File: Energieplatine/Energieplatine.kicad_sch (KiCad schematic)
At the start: 22 parts, among them J1 USB_C_Receptacle_PowerOnly_6P, J2 Conn_01x02_Pin, U1 4027, U2 TL072, U3 LM2576HVT-ADJ, U4 LM2577T-ADJ

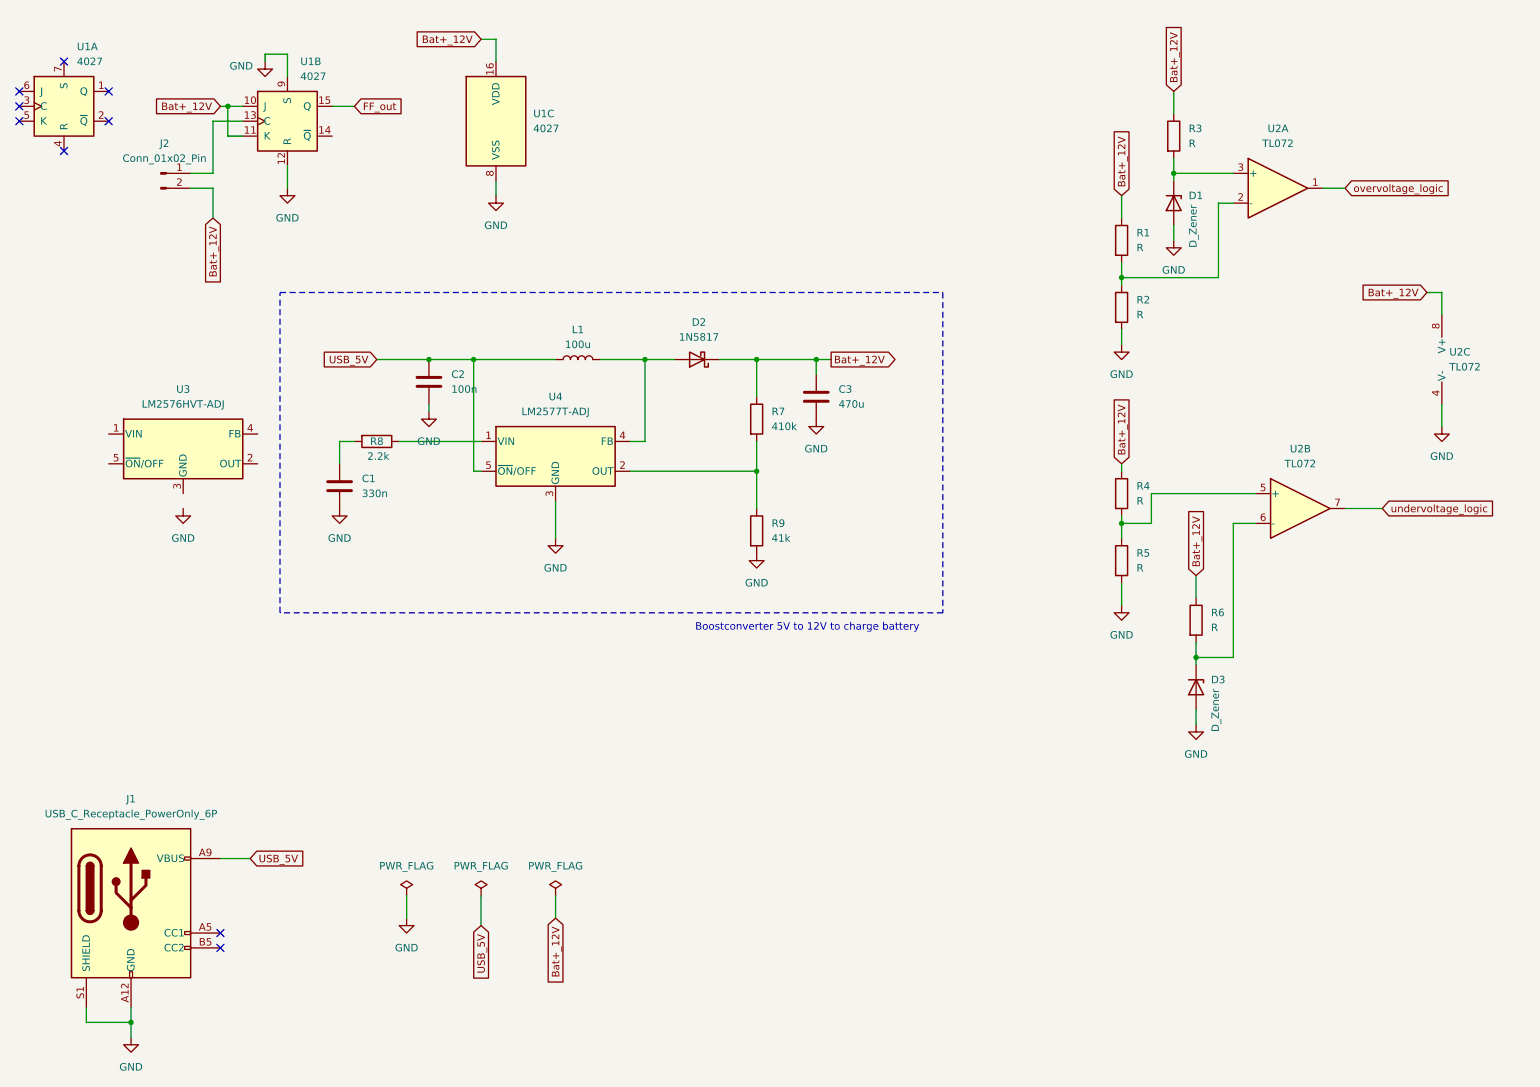
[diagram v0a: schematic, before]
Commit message: Update Energieplatine.kicad_sch
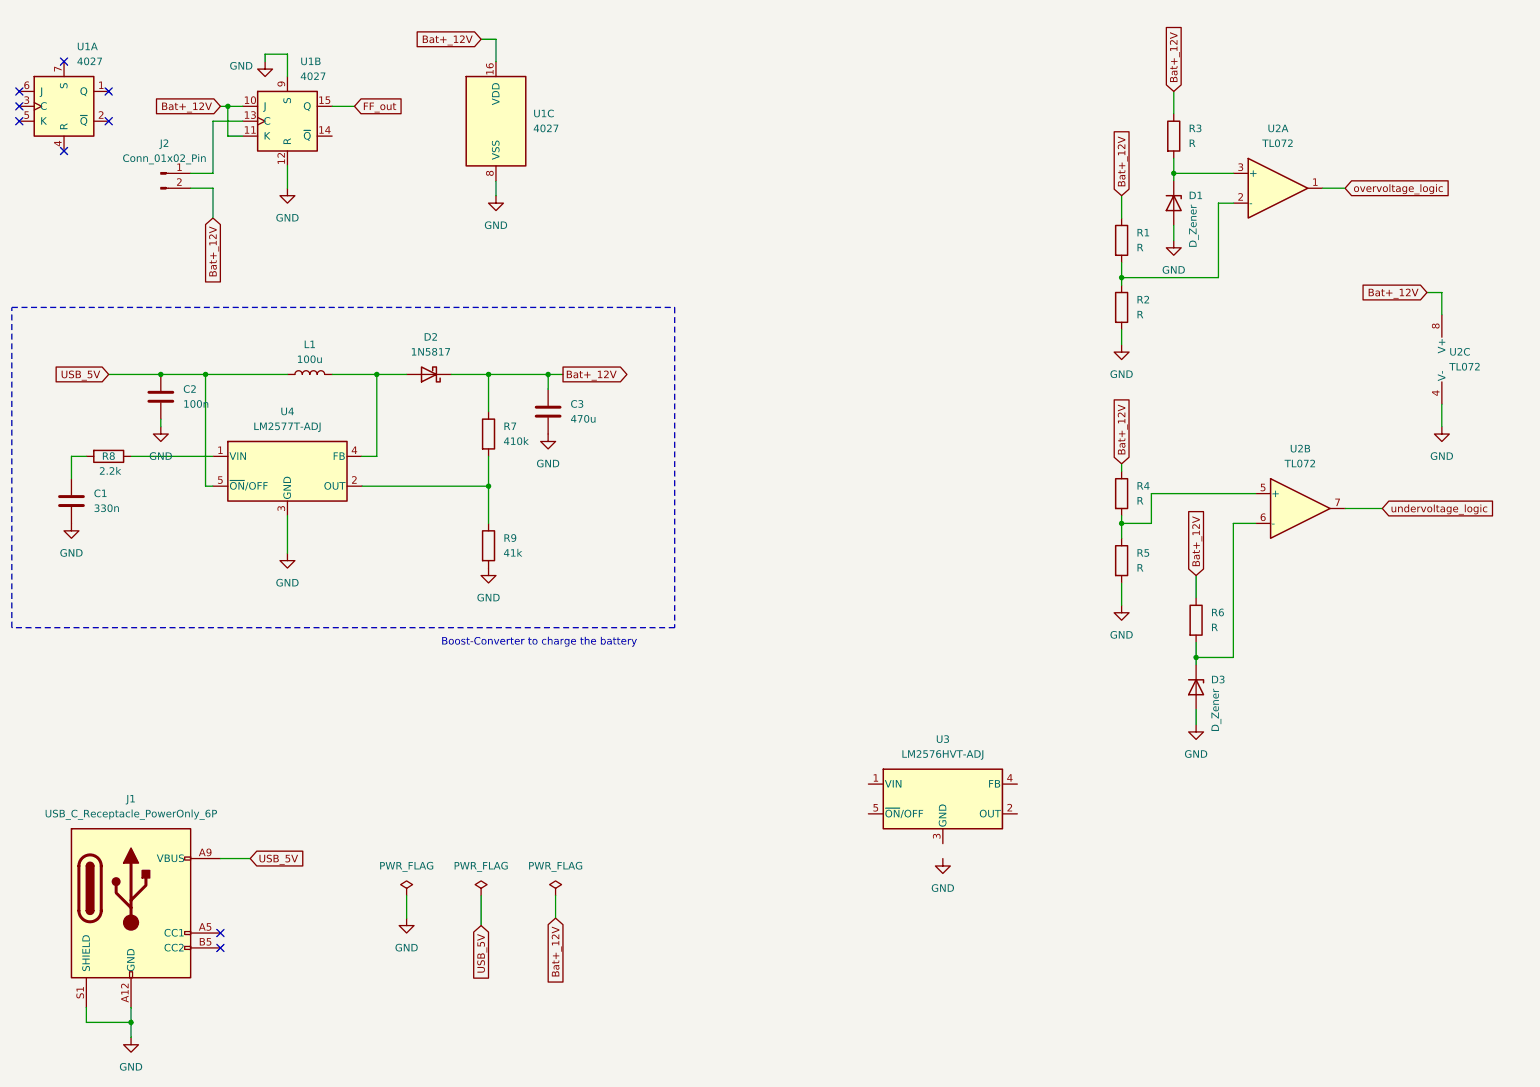
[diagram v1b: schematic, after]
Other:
- note added: "Boost-Converter to charge the battery"
- note removed: "Boostconverter 5V to 12V to charge battery"
- moved on the sheet: C1, C2, C3, D2, L1, R7, R8, R9, U3, U4
